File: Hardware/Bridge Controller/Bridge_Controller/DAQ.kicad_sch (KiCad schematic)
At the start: 24 parts, among them J5 SMA-J-P-H-ST-EM1, J6 SMA-J-P-H-ST-EM1, U6 ADS1118IDGS, U7 AD9833xRM, U8 LMV358, U9 DAC8532

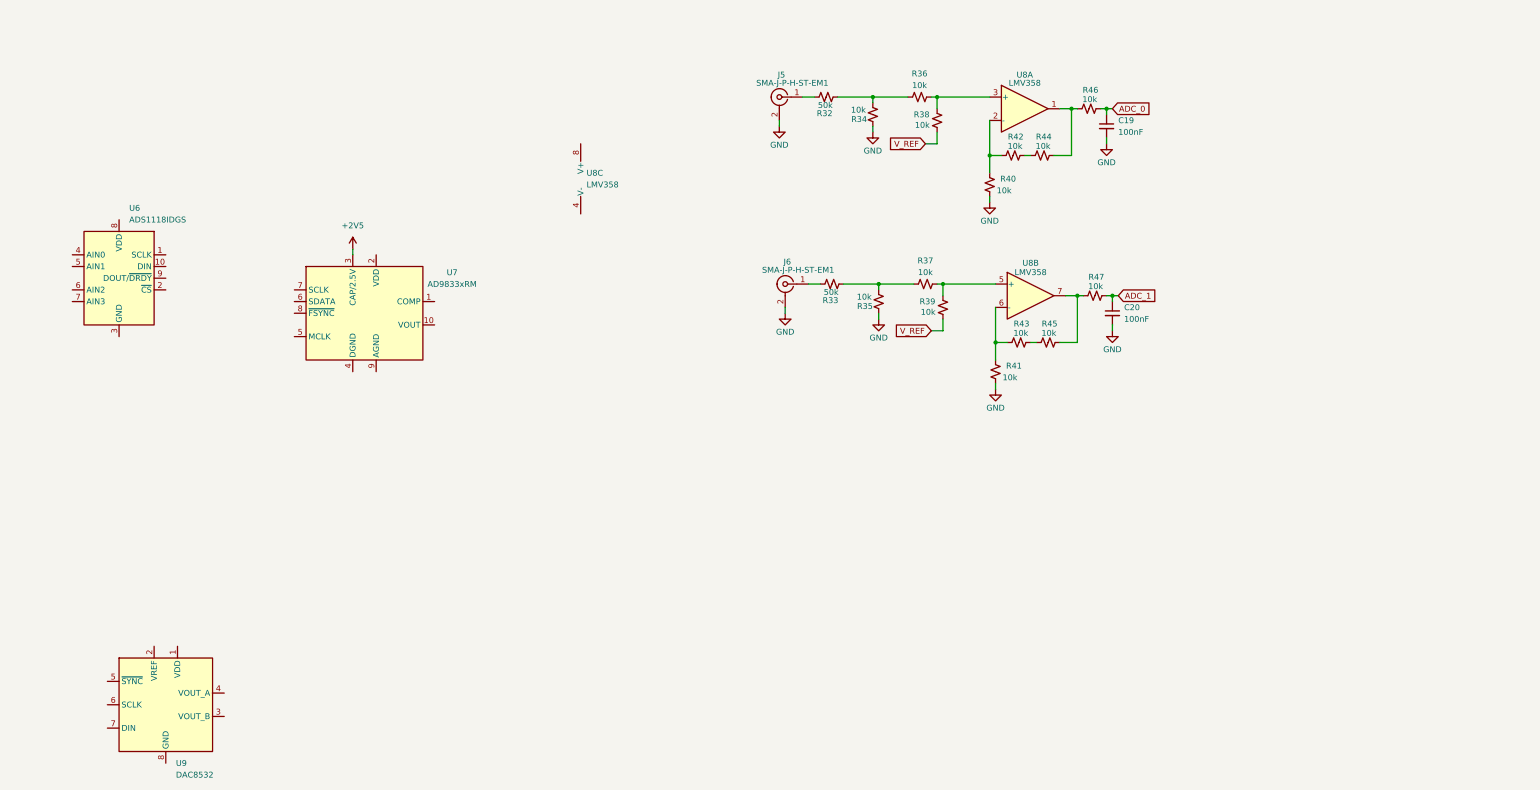
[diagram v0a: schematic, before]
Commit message: Updates to bridge controller
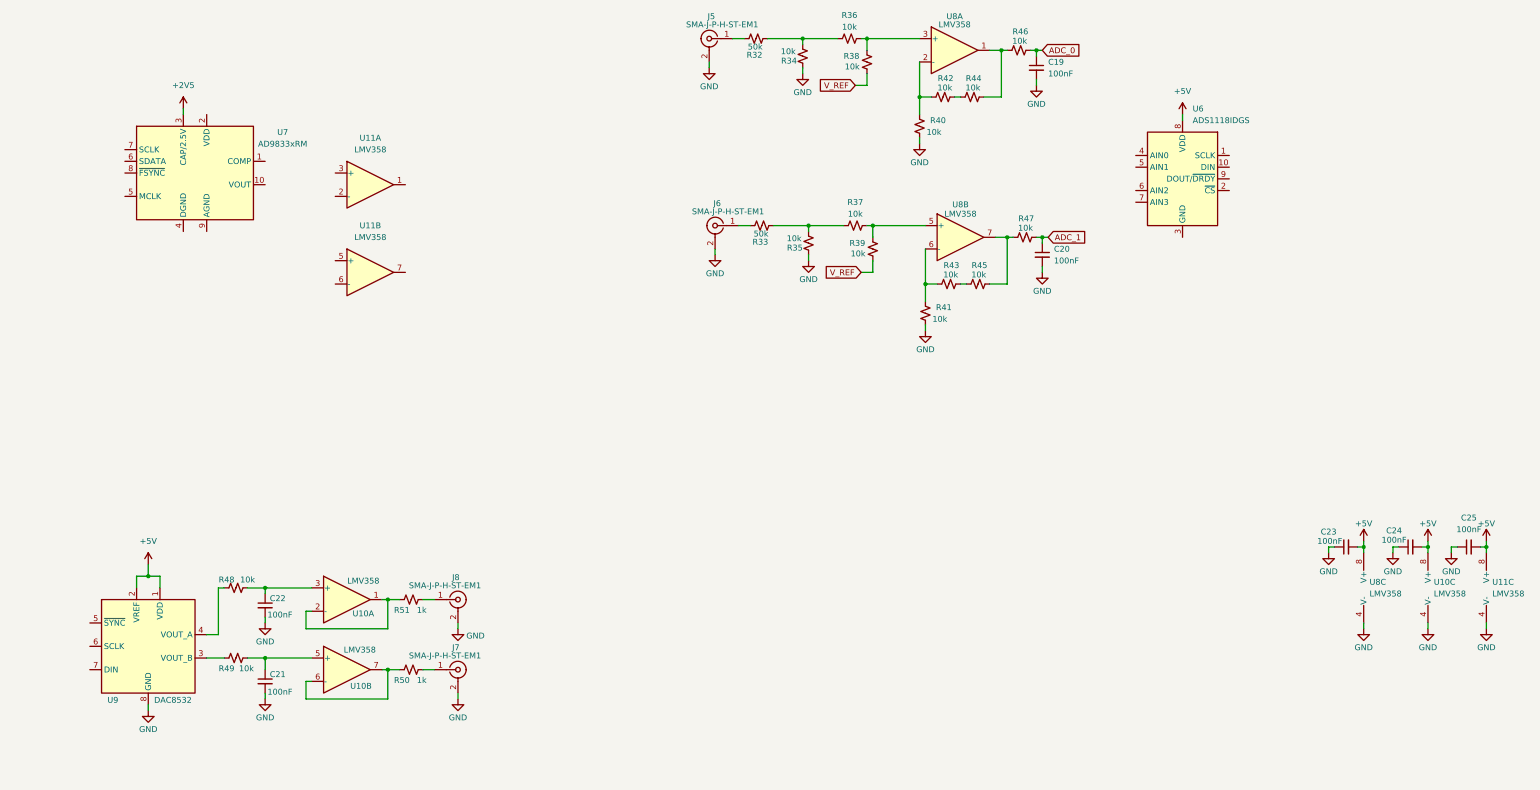
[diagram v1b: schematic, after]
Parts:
- added C21, C22, C23, C24, C25: 100nF, symbol Device:C_Small
- added J7, J8: SMA-J-P-H-ST-EM1, Connector_Coaxial:SMA_Samtec_SMA-J-P-X-ST-EM1_EdgeMount, symbol Connector:Conn_Coaxial
- added R48, R49: 10k, symbol Device:R_Small_US
- added R50, R51: 1k, symbol Device:R_Small_US
- added U10, U11: LMV358, symbol Amplifier_Operational:LMV358
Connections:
- net GND: now also U8.4 (V-), U9.8 (GND), C21.2, C22.2, C23.1, C24.1, C25.1, J7.2 (Ext), J8.2 (Ext), U10.4 (V-), U11.4 (V-)
- net +5V: now reaches U8.8 (V+)
- net +5V: now also U6.8 (VDD), U9.1 (VDD), U9.2 (VREF), C23.2, C24.2, C25.2, U10.8 (V+), U11.8 (V+)
- net at U9.3 (VOUT_B): now also R49.1
- net at U9.4 (VOUT_A): now also R48.1
- new net: C22.1, R48.2, U10.3 (+)
- new net: R51.1, U10.1, U10.2 (-)
- new net: J8.1 (In), R51.2
- new net: C21.1, R49.2, U10.5 (+)
- new net: R50.1, U10.6 (-), U10.7
- new net: J7.1 (In), R50.2
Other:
- moved on the sheet: C19, C20, J5, J6, R32, R33, R34, R35, R36, R37, R38, R39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

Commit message: Updating DAQ
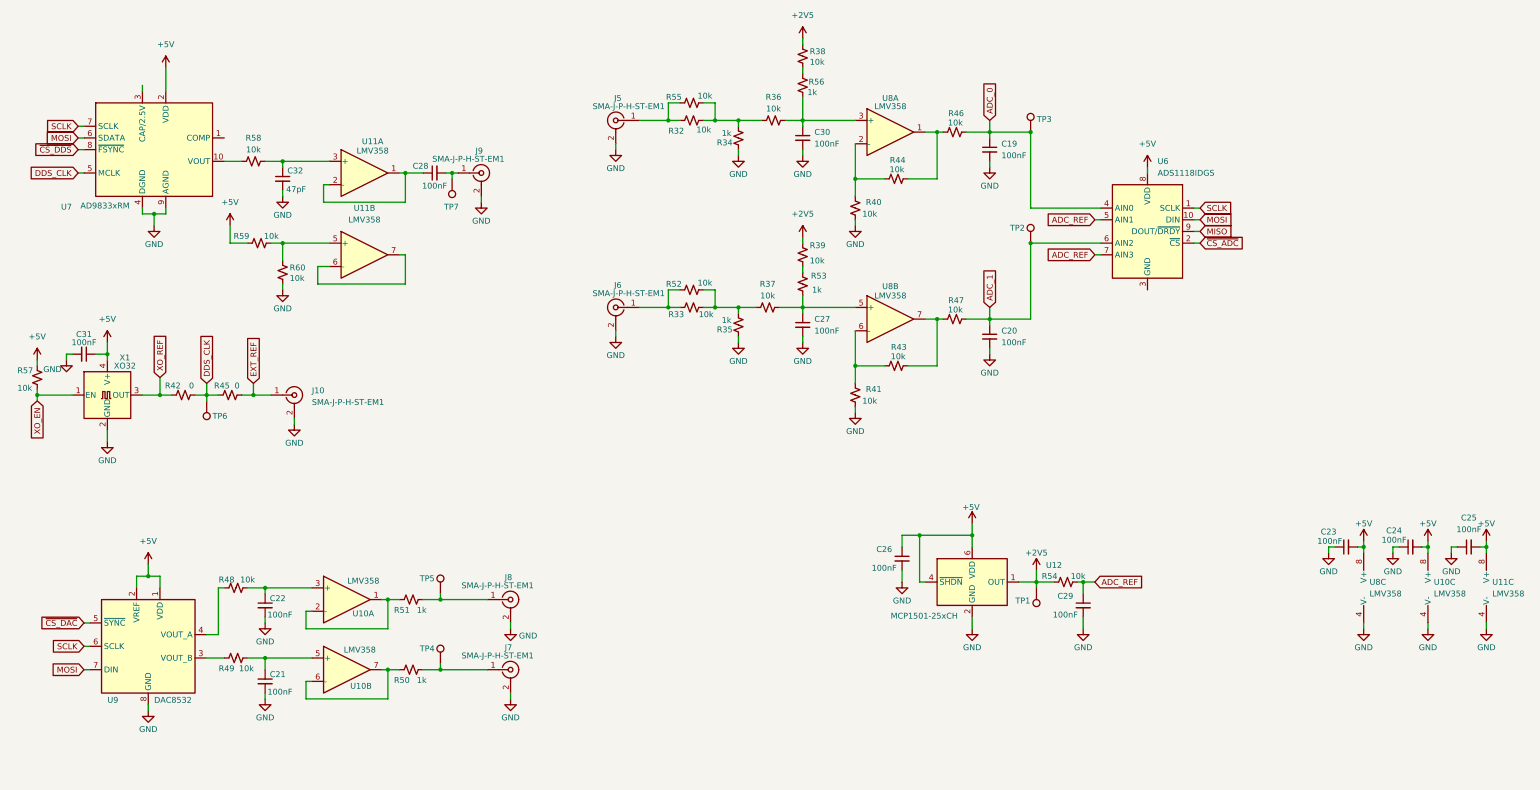
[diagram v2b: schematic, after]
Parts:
- added C26, C27, C28, C29, C30: 100nF, symbol Device:C_Small
- added C31: 100nF, Capacitor_SMD:C_0402_1005Metric, symbol Device:C_Small
- added C32: 47pF, Capacitor_SMD:C_0402_1005Metric, symbol Device:C_Small
- added J10, J9: SMA-J-P-H-ST-EM1, Connector_Coaxial:SMA_Samtec_SMA-J-P-X-ST-EM1_EdgeMount, symbol Connector:Conn_Coaxial
- added R52, R54, R55, R57, R58, R59, R60: 10k, symbol Device:R_Small_US
- added R53: 1k, Resistor_SMD:R_0603_1608Metric, symbol Device:R_Small_US
- added R56: 1k, symbol Device:R_Small_US
- added TP1, TP2, TP3, TP4, TP5, TP6, TP7: TestPoint, symbol Connector:TestPoint
- added U12: MCP1501-25xCH, Package_TO_SOT_SMD:SOT-23-6, symbol Reference_Voltage:MCP1501-25xCH
- added X1: XO32, Oscillator:Oscillator_SMD_EuroQuartz_XO32-4Pin_3.2x2.5mm, symbol Oscillator:XO32
- R32, R33: value 50k -> 10k
- R34, R35: value 10k -> 1k
- R42, R45: value 10k -> 0; footprint (none) -> Resistor_SMD:R_0603_1608Metric
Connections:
- net +2V5: now also R38.2, R39.2, R54.2, TP1.1, U12.1 (OUT); no longer U7.3 (CAP/2.5V)
- net +5V: now also U7.2 (VDD), C26.1, C31.1, R57.2, R59.1, U12.4 (~{SHDN}), U12.6 (VDD), X1.4 (V+)
- net ADC_0: now also U6.4 (AIN0), TP3.1
- net ADC_1: now also U6.6 (AIN2), TP2.1
- net GND: now also U7.4 (DGND), U7.9 (AGND), C26.2, C27.2, C29.2, C30.2, C31.2, C32.2, J10.2 (Ext), J9.2 (Ext), R60.1, U12.2 (GND), U12.3 (GND), U12.5 (GND), X1.2 (GND)
- net at J5.1 (In), R32.1: now also R55.1
- net at R32.2, R34.1, R36.1: now also R55.2
- net at R47.2, U8.7: now also R43.1; no longer R45.1
- net at R44.2: now also R40.2, U8.2 (-); no longer R42.1
- net at R37.2, U8.5 (+): now also C27.1, R53.2; no longer R39.2
- net at J8.1 (In), R51.2: now also TP5.1
- net at U11.5 (+): now also R59.2, R60.2
- net at U11.6 (-): now also U11.7
- net at R33.2, R35.1, R37.1: now also R52.2
- net at U7.10 (VOUT): now also R58.1
- net DDS_CLK: now reaches U7.5 (MCLK)
- net DDS_CLK: now also R42.2, R45.2, TP6.1
- net MOSI: now reaches U7.6 (SDATA)
- net MOSI: now also U6.10 (DIN), U9.7 (DIN)
- net SCLK: now reaches U7.7 (SCLK)
- net SCLK: now also U6.1 (SCLK), U9.6 (SCLK)
- net ~{CS_DDS}: now reaches U7.8 (~{FSYNC})
- net at R36.2, U8.3 (+): now also C30.1, R56.1; no longer R38.2
- net ~{CS_ADC}: now reaches U6.2 (~{CS})
- net ADC_REF: now reaches U6.5 (AIN1)
- net ADC_REF: now also U6.7 (AIN3), C29.1, R54.1
- net MISO: now reaches U6.9 (DOUT/~{DRDY})
- net at U11.1: now also U11.2 (-), C28.1
- net at U11.3 (+): now also C32.1, R58.2
- net at J7.1 (In), R50.2: now also TP4.1
- net at J6.1 (In), R33.1: now also R52.1
- net ~{CS_DAC}: now reaches U9.5 (~{SYNC})
- net V_REF: no longer names the net of R38.1
- net V_REF: now also R56.2; no longer R39.1
- new net: C28.2, J9.1 (In), TP7.1
- new net: R39.1, R53.1
- new net EXT_REF: J10.1 (In), R45.1
- new net XO_EN: R57.1, X1.1 (EN)
- new net XO_REF: R42.1, X1.3 (OUT)
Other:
- moved on the sheet: C19, C20, J5, J6, J7, J8, R32, R33, R34, R35, R36, R37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
